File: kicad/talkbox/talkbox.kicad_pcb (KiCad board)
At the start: 2 copper layers, 89 x 46 mm, 45 parts, among them J1 AudioJack2, J2 Conn_01x02, J3 AudioJack2, J4 Barrel_Jack_Switch, SW1 SW_SPST, U1 LM386, U2 SW_3PDT, U3 TL071, U4 LT1054xSOIC16, U5 LM7812_TO220, U6 LM7912_TO220

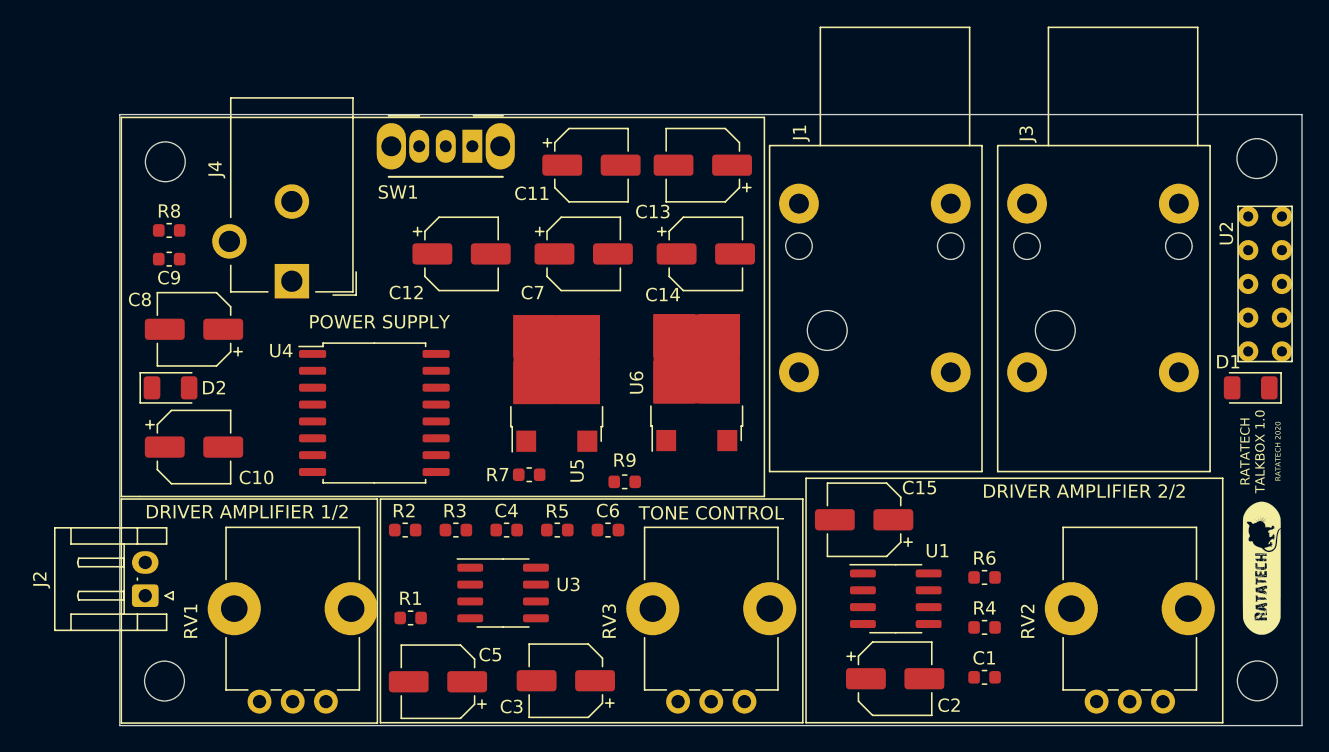
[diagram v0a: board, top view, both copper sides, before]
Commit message: First time routing
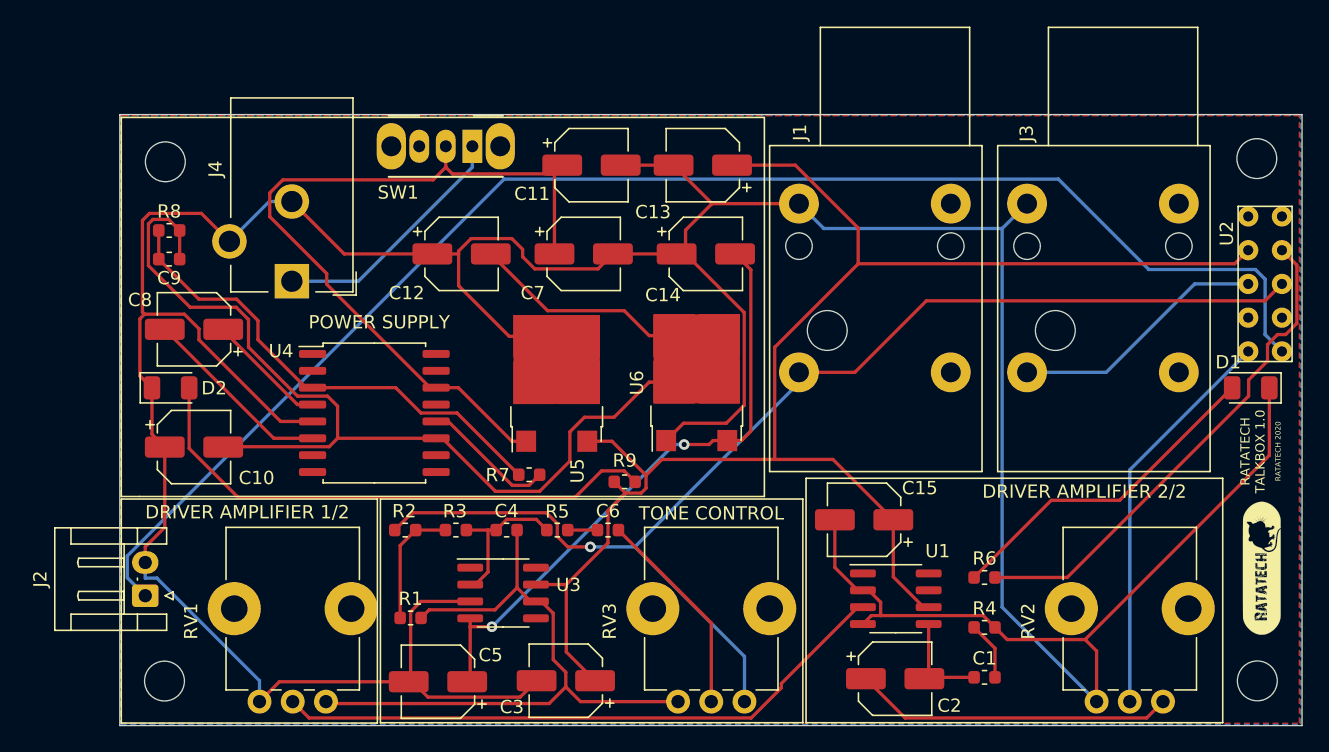
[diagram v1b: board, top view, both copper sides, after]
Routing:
- net GND: track 0.00 -> 311.7 mm
- net VCC: track 0.00 -> 118.7 mm
- net Net-(J2-Pad1): track 0.00 -> 110.0 mm
- net Net-(C10-Pad2): track 0.00 -> 97.8 mm
- net input: track 0.00 -> 92.7 mm, vias 0 -> 1
- net Net-(C11-Pad1): track 0.00 -> 59.5 mm
- net tone_control_output: track 0.00 -> 49.5 mm
- net Net-(RV1-Pad2): track 0.00 -> 47.1 mm
- net VDD: track 0.00 -> 45.9 mm, vias 0 -> 2
- net Net-(D2-Pad2): track 0.00 -> 40.8 mm
- net Net-(R6-Pad2): track 0.00 -> 38.1 mm
- net Net-(C9-Pad2): track 0.00 -> 36.8 mm
- net output: track 0.00 -> 30.1 mm
- net Net-(D1-Pad2): track 0.00 -> 25.3 mm
- net Net-(C2-Pad1): track 0.00 -> 24.1 mm
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- added copper zone on B.Cu, net GND
- added copper zone on F.Cu, net GND
